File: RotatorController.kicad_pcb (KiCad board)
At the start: 2 copper layers, 100 x 70.9 mm, 59 parts, among them J1 USB_A, J2 26 VAC, J3 Rotator, J4 Motor Cap, K1 G5LE-1, K2 G5LE-1, K3 G5LE-1, Q1 BSS123, Q2 BSS123, Q3 BSS123, SW1 SW_CW, SW2 SW_CCW, U1 Teensy4.0, U3 AP2161W

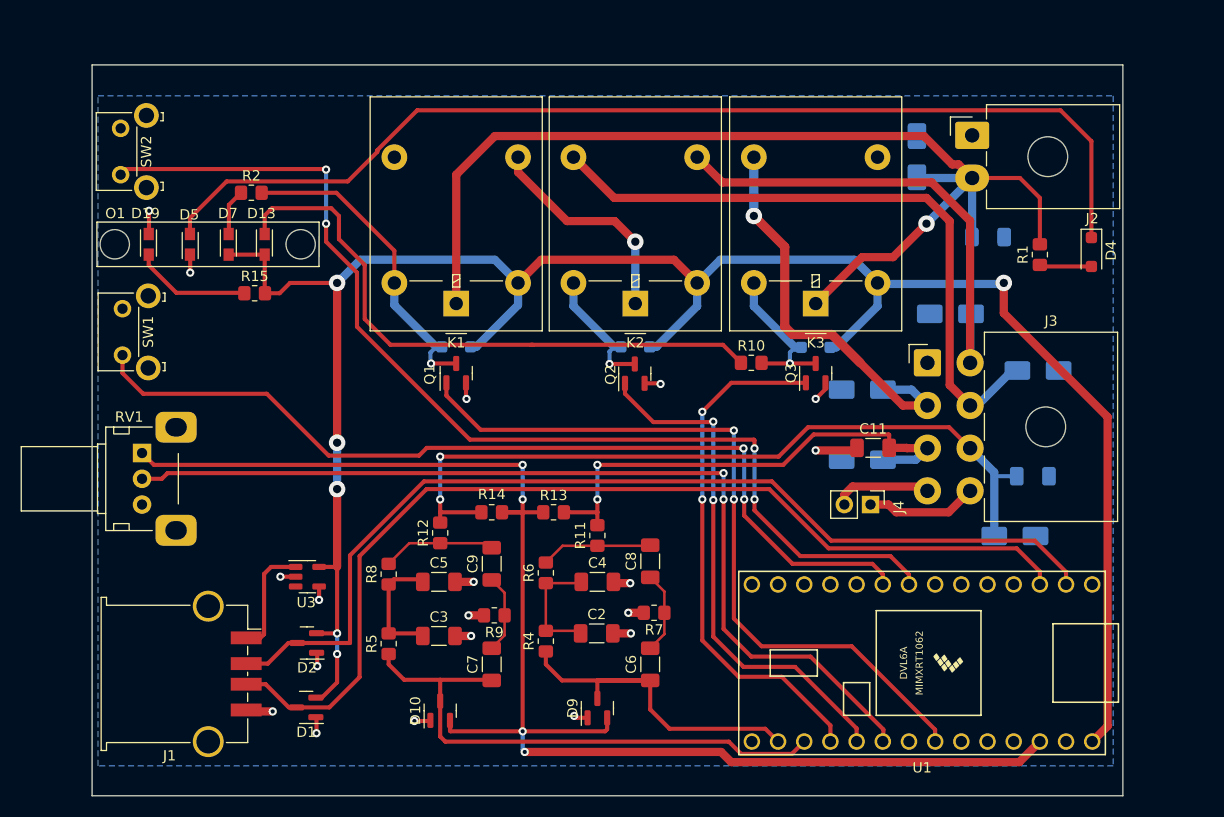
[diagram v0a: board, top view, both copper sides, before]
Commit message: Homing in on final release add ground to pot and button mounting pads added start of dimensions and front panel sketch
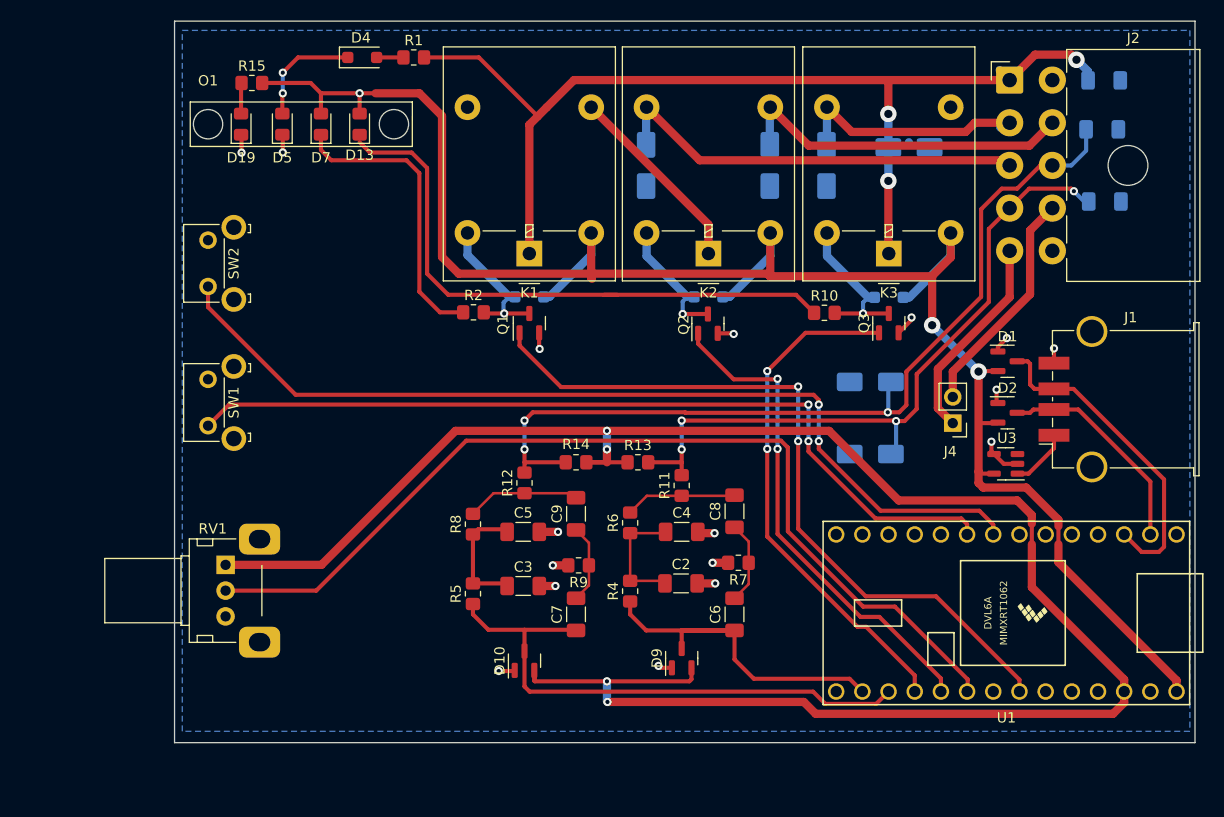
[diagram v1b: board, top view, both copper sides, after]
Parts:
- removed J3: Rotator, Connector_TE-Connectivity:TE_MATE-N-LOK_1-770970-x_2x04_P4.14mm_Horizontal
- C11: moved to B.Cu
- D13, D19, D5, D7: footprint LED_SMD:LED_miniPLCC_2315_Handsoldering -> LED_SMD:LED_0805_2012Metric_Pad1.15x1.40mm_HandSolder
- J2: value 26 VAC -> Rotator; footprint Connector_TE-Connectivity:TE_MATE-N-LOK_1-770966-x_1x02_P4.14mm_Horizontal -> Connector_TE-Connectivity:TE_MATE-N-LOK_1-770971-x_2x05_P4.14mm_Horizontal
- RV1: value R_Potentiometer_US -> Az_Preset
- SW1: value SW_CW -> CW
- SW2: value SW_CCW -> CCW
- moved J1 94.9 mm to (186.7, 91.7), turned to 90 degrees
- moved D1 75.9 mm to (175.8, 88.0), turned to 0 degrees
- moved D4 73.2 mm to (113.2, 58.5), turned to 0 degrees
- moved D2 71.5 mm to (175.8, 93.0), turned to 0 degrees
- moved U3 68.6 mm to (175.6, 98.0), turned to 180 degrees
- moved R1 63.7 mm to (118.2, 58.5), turned to 0 degrees
- moved D17 42.9 mm to (140.8, 69.0), turned to 90 degrees
- moved C12 34.3 mm to (185.0, 65.5)
- moved C11 32.8 mm to (185.2, 72.5), turned to 180 degrees
- moved R2 24.5 mm to (124.0, 83.2)
- moved D18 22.7 mm to (152.8, 69.0), turned to 90 degrees
- moved D16 22.0 mm to (158.2, 69.0), turned to 90 degrees
- moved D15 20.5 mm to (162.5, 90.0), turned to 0 degrees
- moved R15 20.4 mm to (102.5, 61.0)
- moved C1 18.9 mm to (185.2, 60.8)
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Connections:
- J2 pad 1: GND -> /26VAC
- J2 pad 2: /26VAC -> /Brake
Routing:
- net Net-(D4-K): track 104.0 -> 10.9 mm, vias 0 -> 2
- net /Ctlr_Rx: track 96.8 -> 21.1 mm
- net /Ctlr_Tx: track 98.2 -> 32.6 mm
- net /3V3: track 140.5 -> 189.1 mm
- net Net-(D7-K): track 4.50 -> 28.6 mm
- net /+5V: track 204.9 -> 182.3 mm, vias 6 -> 3
- net /Right: track 63.8 -> 41.2 mm
- net /Wiper+: track 48.6 -> 68.2 mm, vias 2 -> 4
- net /Brake: track 39.7 -> 23.1 mm, vias 1 -> 0
- net Net-(D6-A): track 30.4 -> 14.2 mm
- net /CCW: track 105.1 -> 90.7 mm, vias 4 -> 2
- net /Left: track 47.6 -> 34.0 mm
- net /Cap1: track 9.52 -> 22.3 mm
- net /Wiper-: track 75.5 -> 86.4 mm, vias 2 -> 3
- net /Cap2: track 10.8 -> 20.2 mm
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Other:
- board size 100 x 70.9 mm -> 99 x 70 mm
